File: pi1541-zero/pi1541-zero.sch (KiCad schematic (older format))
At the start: 1 part, among them J1 RPi_GPIO

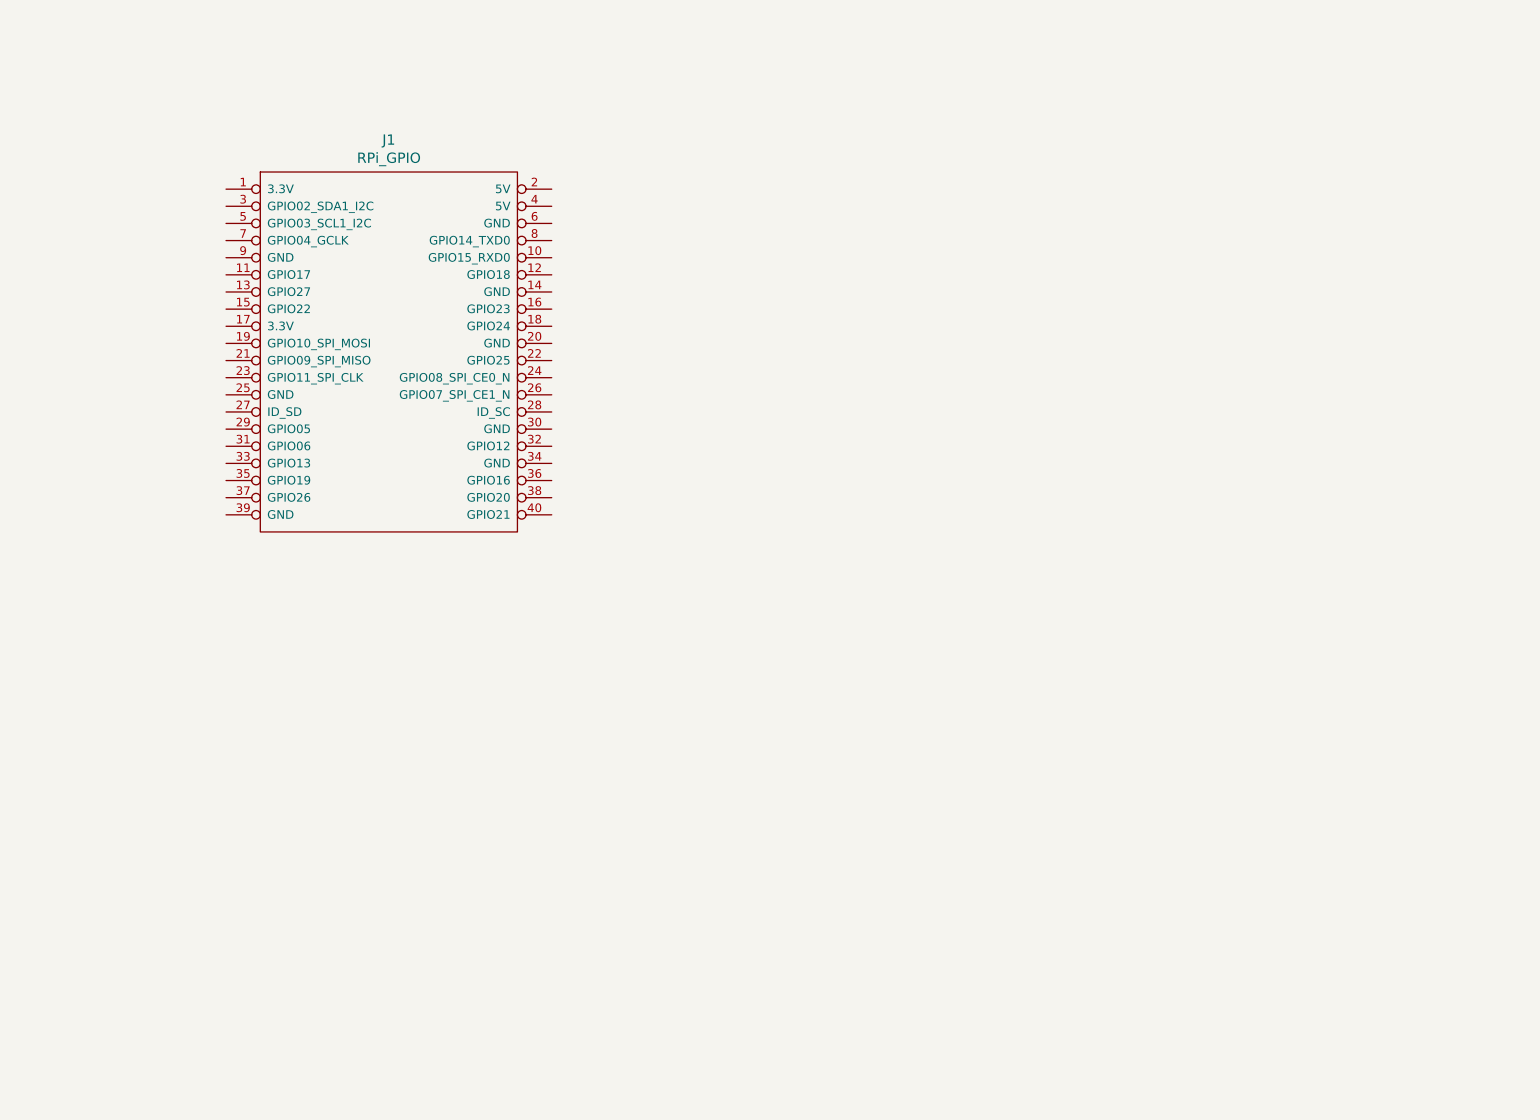
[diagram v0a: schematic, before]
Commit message: first draft
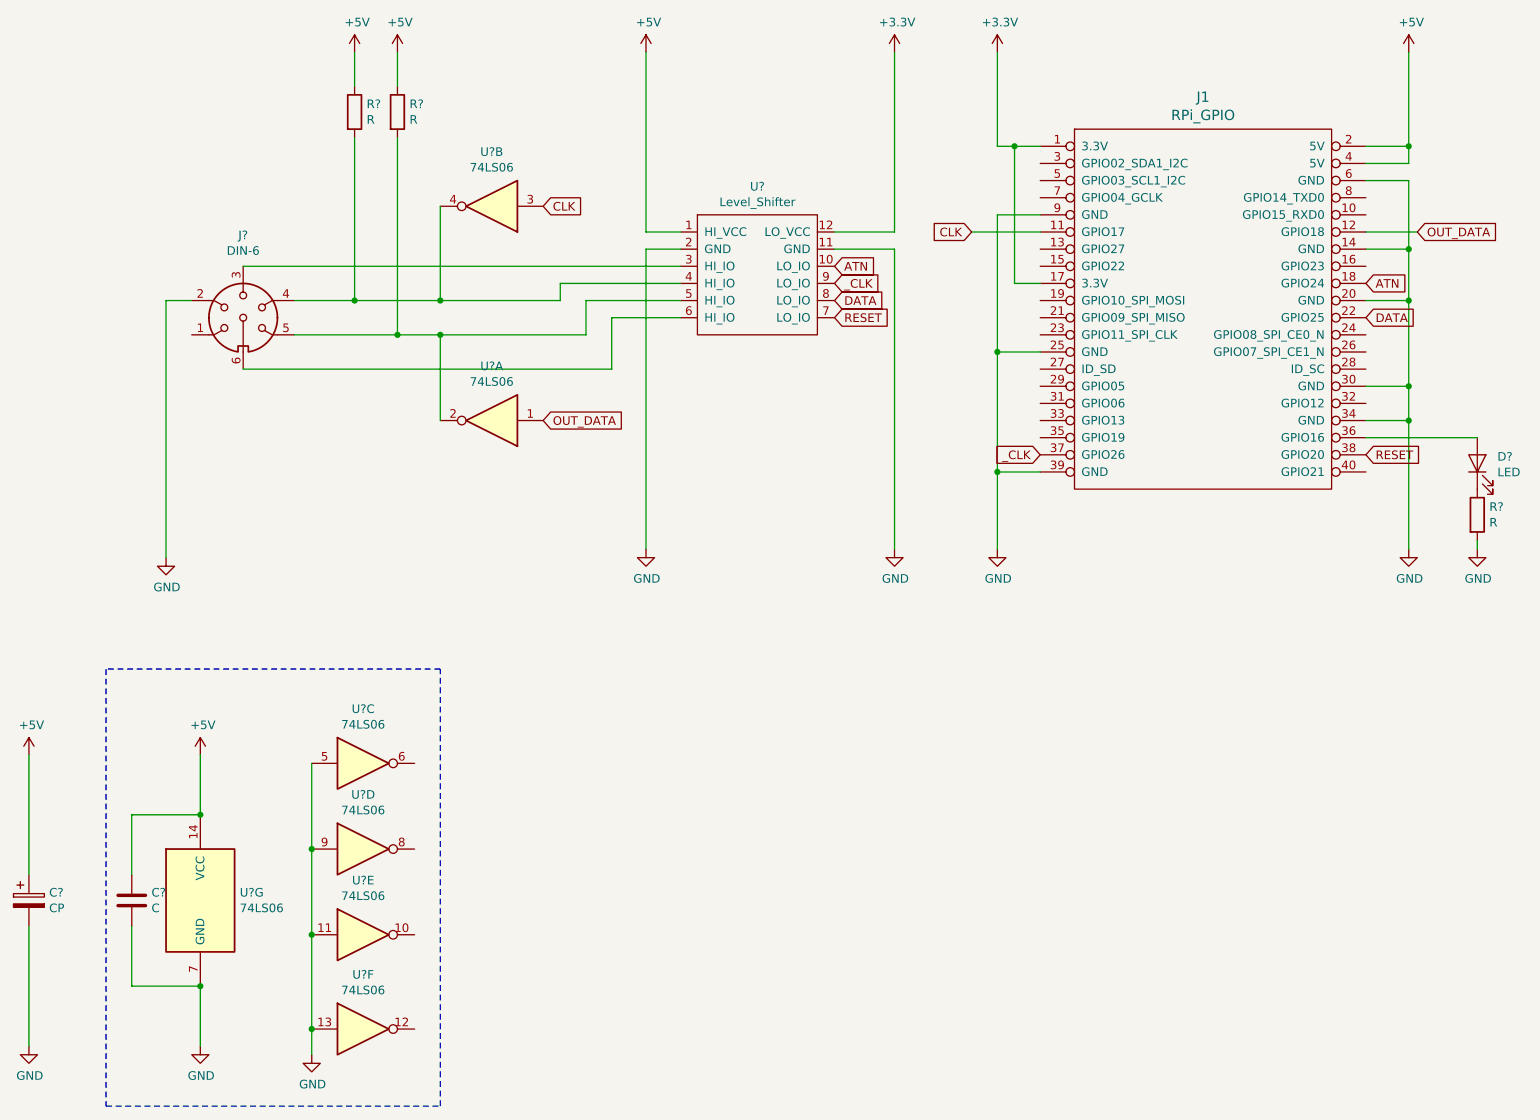
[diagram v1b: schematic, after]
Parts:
- added C?: CP, symbol Device:CP
- added C?: C, symbol Device:C
- added D?: LED, symbol Device:LED
- added J?: DIN-6, symbol Connector:DIN-6
- added R? (x3): R, symbol Device:R
- added U?: Level_Shifter, symbol pi1541:Level_Shifter
- added U? (x7): 74LS06, symbol 74xx:74LS06
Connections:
- net +3V3: now reaches J1.1 (3.3V)
- net +3V3: now also J1.17 (3.3V), U?.12 (LO_VCC)
- net CLK: now reaches J1.11 (GPIO17)
- net CLK: now also U?.3
- net OUT_DATA: now reaches J1.12 (GPIO18)
- net OUT_DATA: now also U?.1
- net GND: now reaches J1.14 (GND)
- net GND: now also J1.20 (GND), J1.25 (GND), J1.30 (GND), J1.34 (GND), J1.39 (GND), J1.6 (GND), J1.9 (GND), C?.2, C?.2, J?.2, R?.2, U?.11, U?.11 (GND), U?.13, U?.2 (GND), U?.5, U?.7 (GND), U?.9
- net ATN: now reaches J1.18 (GPIO24)
- net ATN: now also U?.10 (LO_IO)
- net +5V: now reaches J1.2 (5V)
- net +5V: now also J1.4 (5V), C?.1, C?.1, R?.1, R?.1, U?.1 (HI_VCC), U?.14 (VCC)
- net DATA: now reaches J1.22 (GPIO25)
- net DATA: now also U?.8 (LO_IO)
- net at J1.36 (GPIO16): now also D?.2 (A)
- net _CLK: now reaches J1.37 (GPIO26)
- net _CLK: now also U?.9 (LO_IO)
- net RESET: now reaches J1.38 (GPIO20)
- net RESET: now also U?.7 (LO_IO)
- new net: J?.3, U?.3 (HI_IO)
- new net: J?.4, R?.2, U?.4, U?.4 (HI_IO)
- new net: J?.5, R?.2, U?.2, U?.5 (HI_IO)
- new net: J?.6, U?.6 (HI_IO)
- new net: D?.1 (K), R?.1
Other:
- moved on the sheet: J1
